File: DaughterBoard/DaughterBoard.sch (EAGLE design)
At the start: 10 parts

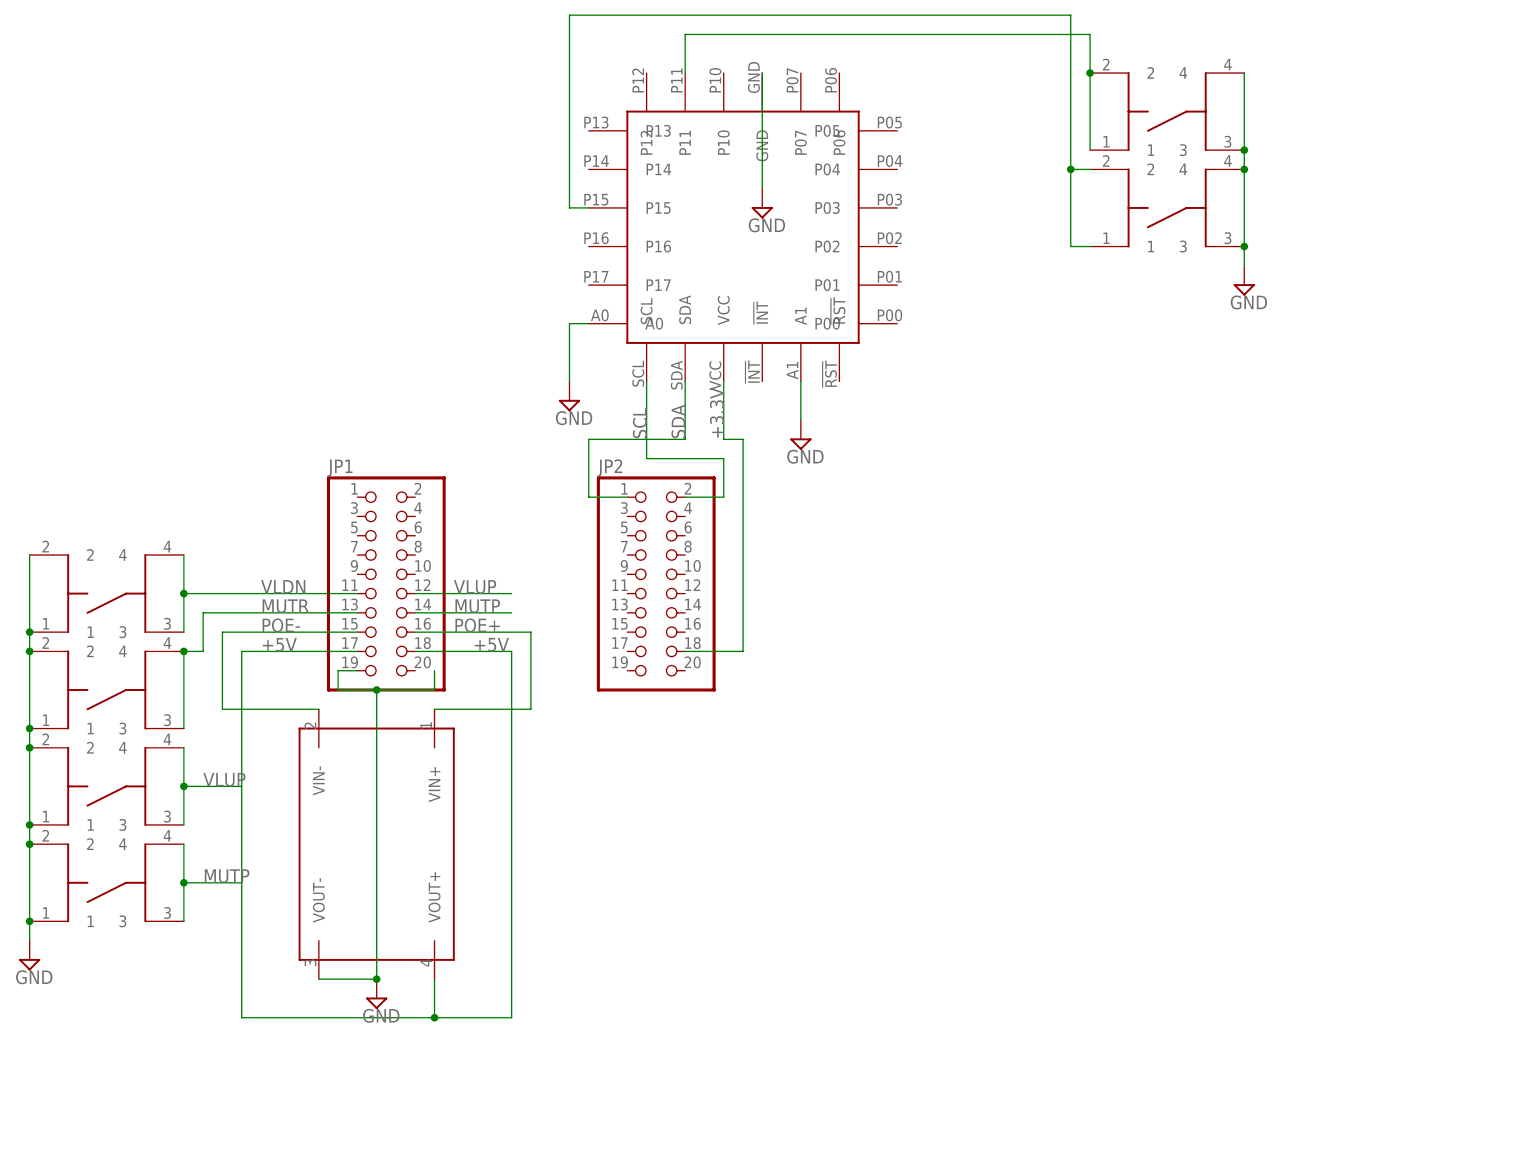
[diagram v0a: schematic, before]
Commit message: Added a motor Driver
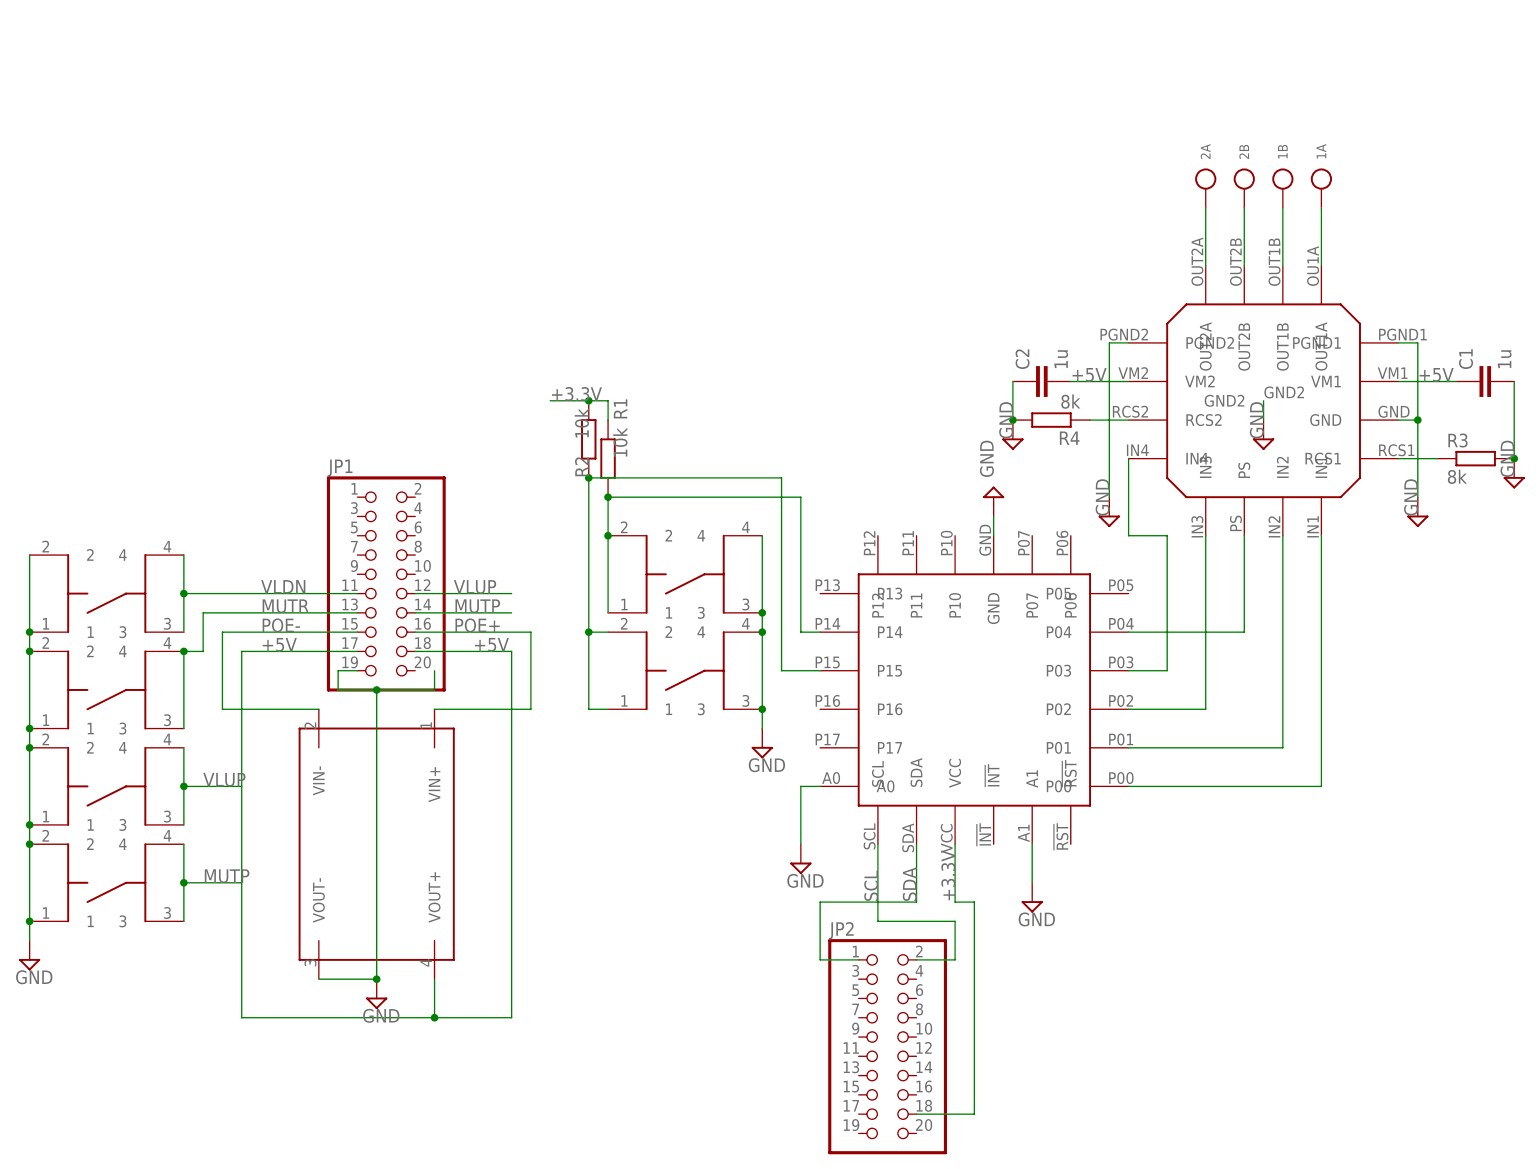
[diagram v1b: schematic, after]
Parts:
- added 1A, 1B, 2A, 2B: TP1R, pm-labs:TP1R
- added C1, C2: 1u, pm-labs:C0603R
- added R1, R2: 10k, pm-labs:R0603R
- added R3, R4: 8k, pm-labs:R0603R
- added U$9: DRIVER_LV8716QA-MH, PiProject:DRIVER_LV8716QA-MH
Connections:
- new net N$10: 2A.1, U$9.OUT2A
- new net N$11: 2B.1, U$9.OUT2B
- new net N$12: 1B.1, U$9.OUT1B
- new net N$13: 1A.1, U$9.OUT1A
- new net N$3: R4.1, U$9.RCS2
- new net N$4: R3.1, U$9.RCS1
- new net N$5: U$6.P00, U$9.IN1
- new net N$6: U$6.P01, U$9.IN2
- new net N$7: U$6.P02, U$9.IN3
- new net N$8: U$6.P03, U$9.IN4
- new net N$9: U$6.P04, U$9.PS
- net +3.3V: now also R1.2, R2.2
- net +5V: now also C1.1, C2.2, U$9.VM1, U$9.VM2
- net GND: now also C1.2, C2.1, R3.2, R4.2, U$9.GND, U$9.GND2, U$9.PGND1, U$9.PGND2
- net N$1: now also R1.1, U$6.P14; no longer U$6.P11
- net N$2: now also R2.1
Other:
- moved on the sheet: JP2
